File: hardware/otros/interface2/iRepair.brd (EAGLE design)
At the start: 72 x 26.1 mm, 12 parts, among them IC4 AM29F040S

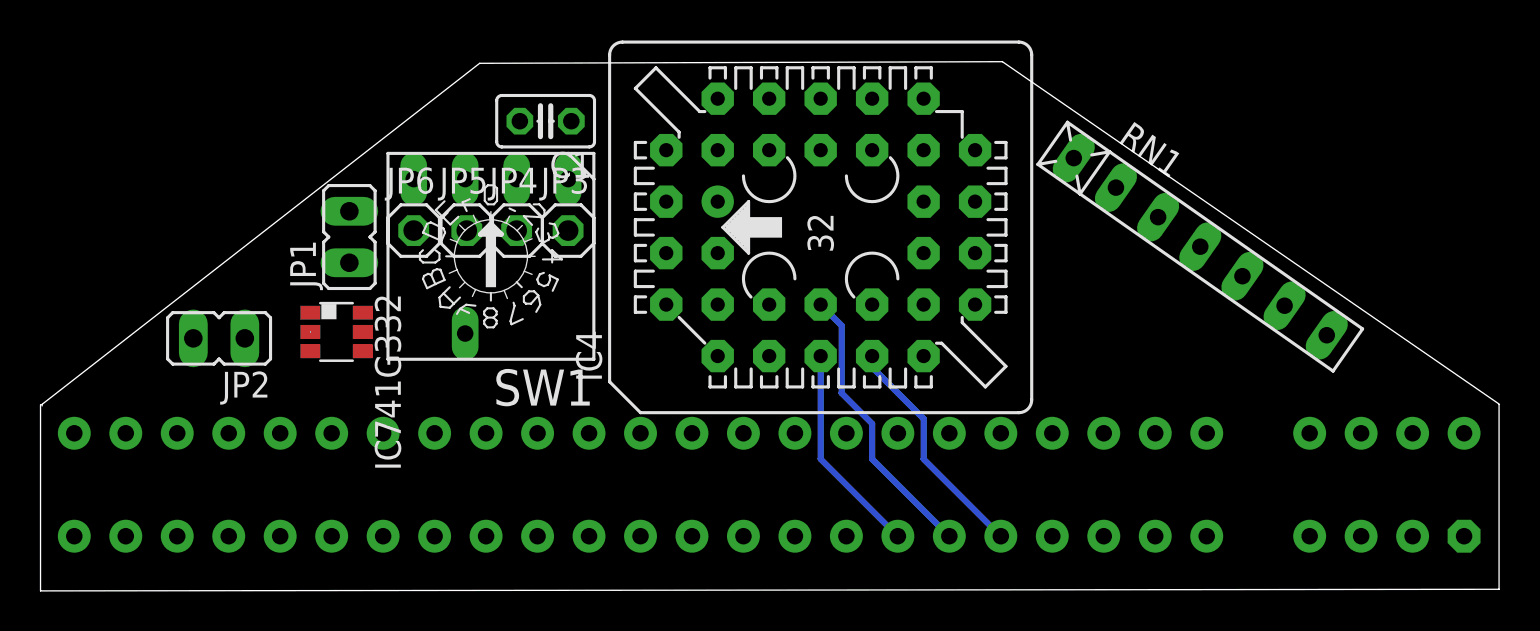
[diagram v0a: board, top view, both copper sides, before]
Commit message: Acabo iRepair
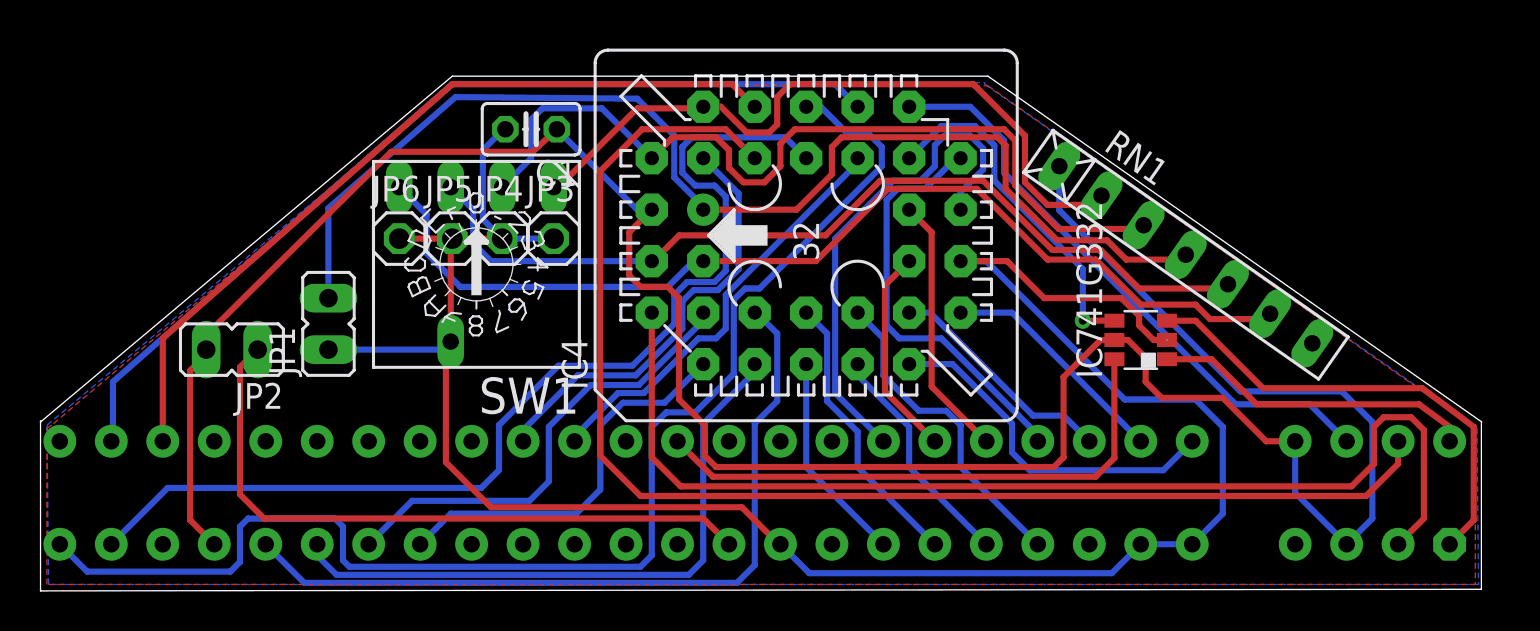
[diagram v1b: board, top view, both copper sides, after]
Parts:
- moved IC741G332 39.7 mm to (54.3, 12.4), turned to 90 degrees
- moved JP1 4.41 mm to (14.2, 13.2)
- moved JP2 0.84 mm to (9.45, 11.9)
- moved U$3 0.82 mm to (69.5, 7.38)
- moved IC4 0.82 mm to (37.8, 17.5)
- moved JP3 0.82 mm to (25.3, 17.4)
- moved JP4 0.82 mm to (22.8, 17.4)
- moved JP5 0.82 mm to (20.3, 17.4)
- moved JP6 0.82 mm to (17.7, 17.4)
- moved SW1 0.82 mm to (21.5, 16.1)
- moved C1 0.82 mm to (24.2, 22.8)
- moved RN1 0.82 mm to (56.5, 16.6)
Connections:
- removed net NMI: U$3.B14
- removed net RESET: U$3.A20
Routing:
- net VCC: track 0.00 -> 125.6 mm
- net GND: track 0.00 -> 105.8 mm
- net A13: track 0.00 -> 65.1 mm
- net A11: track 0.00 -> 64.7 mm
- net N$2: track 0.00 -> 58.5 mm
- net A12: track 0.00 -> 54.7 mm
- net A9: track 0.00 -> 52.3 mm
- net N$5: track 0.00 -> 50.9 mm
- net A10: track 0.00 -> 45.7 mm
- net N$4: track 0.00 -> 44.8 mm
- net N$3: track 0.00 -> 42.4 mm
- net A8: track 0.00 -> 39.5 mm
- net A4: track 0.00 -> 38.7 mm
- net N$6: track 0.00 -> 35.0 mm
- net N$1: track 0.00 -> 32.7 mm
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- added copper zone on layer 1, net GND
- added copper zone on layer 16, net GND
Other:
- board size 72 x 26.1 mm -> 71.1 x 25.4 mm
- board text added: "AntonioVillena sep2016"
- board text removed: "AntonioVillena jul2015"
